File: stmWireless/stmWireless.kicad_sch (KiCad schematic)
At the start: 51 parts, among them IC1 BALFLB-WL-08D3, J1 SWD, J2 CORTEX_DEBUG, J3 Conn_02x08_Top_Bottom, J4 SMA, U1 STM32WLE5CBU6, U2 AP63203WU, U3 BGS12WN6E6327, Y1 Crystal_32MHz, Y2 Crystal_32.768kHz

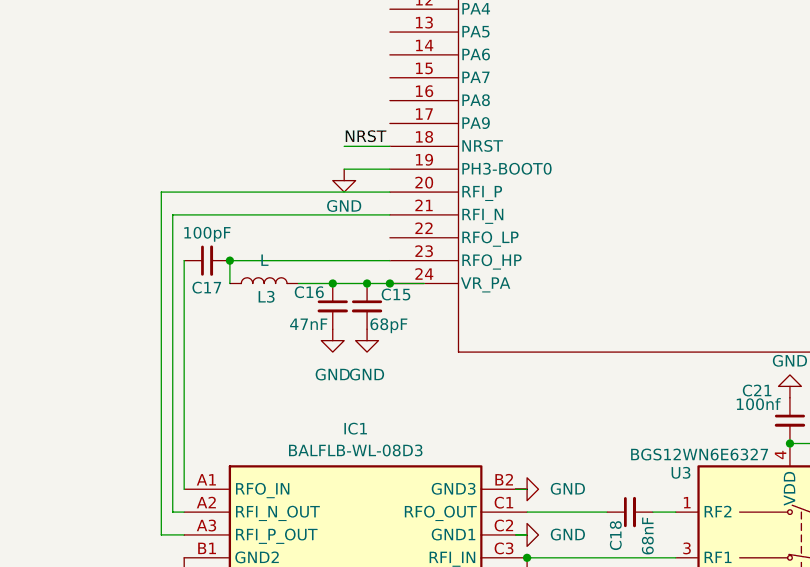
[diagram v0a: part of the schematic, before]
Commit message: assign footprints and minor cleanup
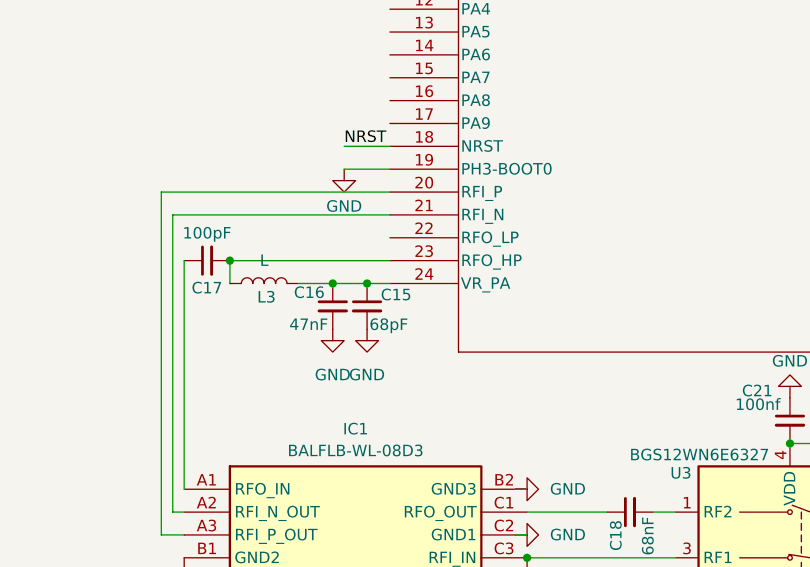
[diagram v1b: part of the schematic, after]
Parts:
- C15, C16, C17, C18, C19, C20, C21, C22, C23, C24, C25, C26, C27: footprint (none) -> Capacitor_SMD:C_0603_1608Metric
- IC1: footprint BALFLBWL08D3 -> Project_library:BALFLBWL08D3
- R7, R8: footprint (none) -> Resistor_SMD:R_0603_1608Metric
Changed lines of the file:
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@@
 	)
 	(junction
-		(at 109.22 129.54)
-		(diameter 0)
-		(color 0 0 0 0)
-	)
-	(junction
 		(at 241.3 68.58)
 		(diameter 0)
@@
 	(wire
 		(pts
-			(xy 113.03 129.54) (xy 109.22 129.54)
-		)
-		(stroke
-			(width 0)
-			(type default)
-		)
-	)
-	(wire
-		(pts
 			(xy 160.02 147.32) (xy 163.83 147.32)
 		)
@@
 			)
 		)
-		(property "Footprint" "BALFLBWL08D3"
+		(property "Footprint" "Project_library:BALFLBWL08D3"
 			(at 120.65 247.32 0)
 			(effects
@@
 			)
 		)
-		(property "Footprint" ""
+		(property "Footprint" "Capacitor_SMD:C_0603_1608Metric"
 			(at 177.8 154.94 0)
 			(effects
@@
 			)
 		)
-		(property "Footprint" ""
+		(property "Footprint" "Capacitor_SMD:C_0603_1608Metric"
 			(at 124.46 162.56 0)
 			(effects
@@
 			)
 		)
-		(property "Footprint" ""
+		(property "Footprint" "Capacitor_SMD:C_0603_1608Metric"
 			(at 153.67 144.78 0)
 			(effects
@@
 			)
 		)
-		(property "Footprint" ""
+		(property "Footprint" "Resistor_SMD:R_0603_1608Metric"
 			(at 167.64 149.098 90)
 			(effects
@@
 			)
 		)
-		(property "Footprint" ""
+		(property "Footprint" "Capacitor_SMD:C_0603_1608Metric"
 			(at 185.42 154.94 0)
 			(effects
@@
 			)
 		)
-		(property "Footprint" ""
+		(property "Footprint" "Capacitor_SMD:C_0603_1608Metric"
 			(at 88.9 127 0)
 			(effects
@@
 			)
 		)
-		(property "Footprint" ""
+		(property "Footprint" "Capacitor_SMD:C_0603_1608Metric"
 			(at 135.89 154.94 0)
 			(effects
@@
 			)
 		)
-		(property "Footprint" ""
+		(property "Footprint" "Capacitor_SMD:C_0603_1608Metric"
 			(at 160.02 184.15 0)
 			(effects
@@
 			)
 		)
-		(property "Footprint" ""
+		(property "Footprint" "Capacitor_SMD:C_0603_1608Metric"
 			(at 106.68 132.08 0)
 			(effects
@@
 			)
 		)
-		(property "Footprint" ""
+		(property "Footprint" "Capacitor_SMD:C_0603_1608Metric"
 			(at 102.87 132.08 0)
 			(effects
@@
 			)
 		)
-		(property "Footprint" ""
+		(property "Footprint" "Capacitor_SMD:C_0603_1608Metric"
 			(at 171.45 184.15 0)
 			(effects
@@
 			)
 		)
-		(property "Footprint" ""
+		(property "Footprint" "Capacitor_SMD:C_0603_1608Metric"
 			(at 133.35 187.96 0)
 			(effects
@@
 			)
 		)
-		(property "Footprint" ""
+		(property "Footprint" "Capacitor_SMD:C_0603_1608Metric"
 			(at 146.05 187.96 0)
 			(effects
@@
 			)
 		)
-		(property "Footprint" ""
+		(property "Footprint" "Capacitor_SMD:C_0603_1608Metric"
 			(at 160.02 144.78 0)
 			(effects
@@
 			)
 		)
-		(property "Footprint" ""
+		(property "Footprint" "Resistor_SMD:R_0603_1608Metric"
 			(at 194.31 154.178 90)
 			(effects
